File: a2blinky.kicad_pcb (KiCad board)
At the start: 2 copper layers, 75 x 75 mm, 25 parts, among them J1 Barrel_Jack_Switch, U1 74HC164, U2 4072, U3 AP1117-33, U4 LMC555xM

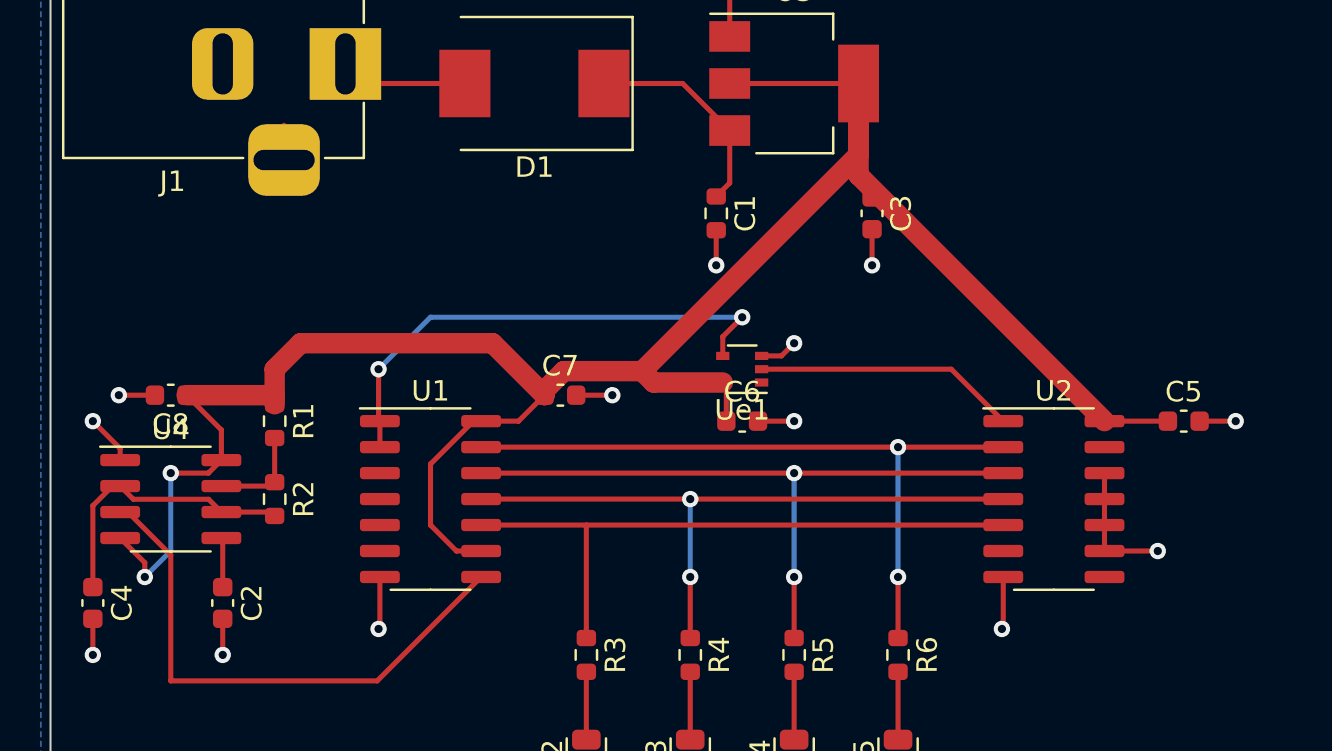
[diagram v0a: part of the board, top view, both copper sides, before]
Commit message: bom
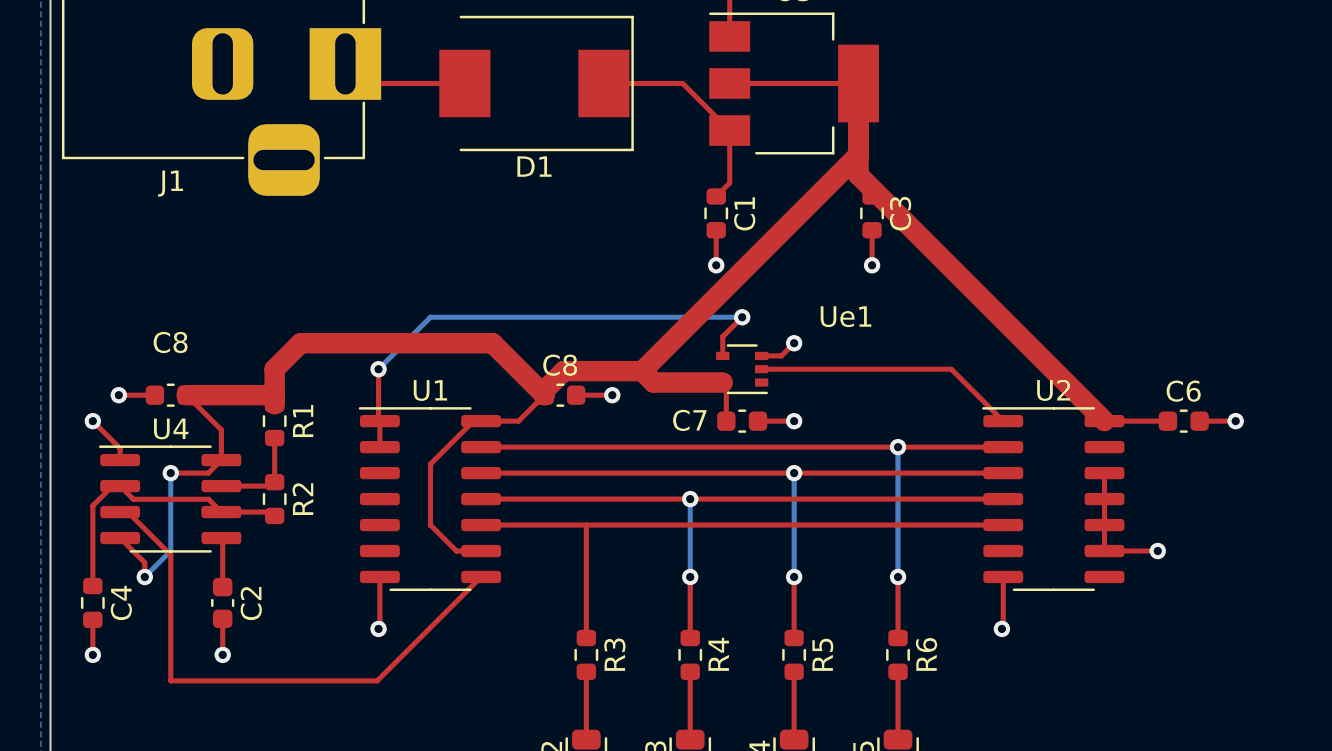
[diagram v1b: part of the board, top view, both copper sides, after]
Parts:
- removed C5: 100n, Capacitor_SMD:C_0603_1608Metric
- added C8: 100n, Capacitor_SMD:C_0603_1608Metric, F.Cu at (74.9, 76.2)
- C3, C4: footprint Capacitor_SMD:C_0603_1608Metric -> Resistor_SMD:R_0603_1608Metric
- moved C6 21.6 mm to (105.4, 77.5)
- moved C7 8.98 mm to (83.8, 77.5)
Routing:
- net GND: track 51.5 -> 49.8 mm
